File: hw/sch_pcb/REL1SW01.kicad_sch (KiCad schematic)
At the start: 22 parts, among them J1 HEADER_2x02_PARALLEL, J2 HEADER_2x02_PARALLEL, J3 HEADER_2x06_PARALLEL, J4 HEADER_2x06_PARALLEL, J5 HEADER_2x04_PARALLEL, M1 SROUB3M, M2 SROUB3M, M3 SROUB3M, M4 SROUB3M, T1 IRLML6244, T2 IRLML6244, X1 RELE

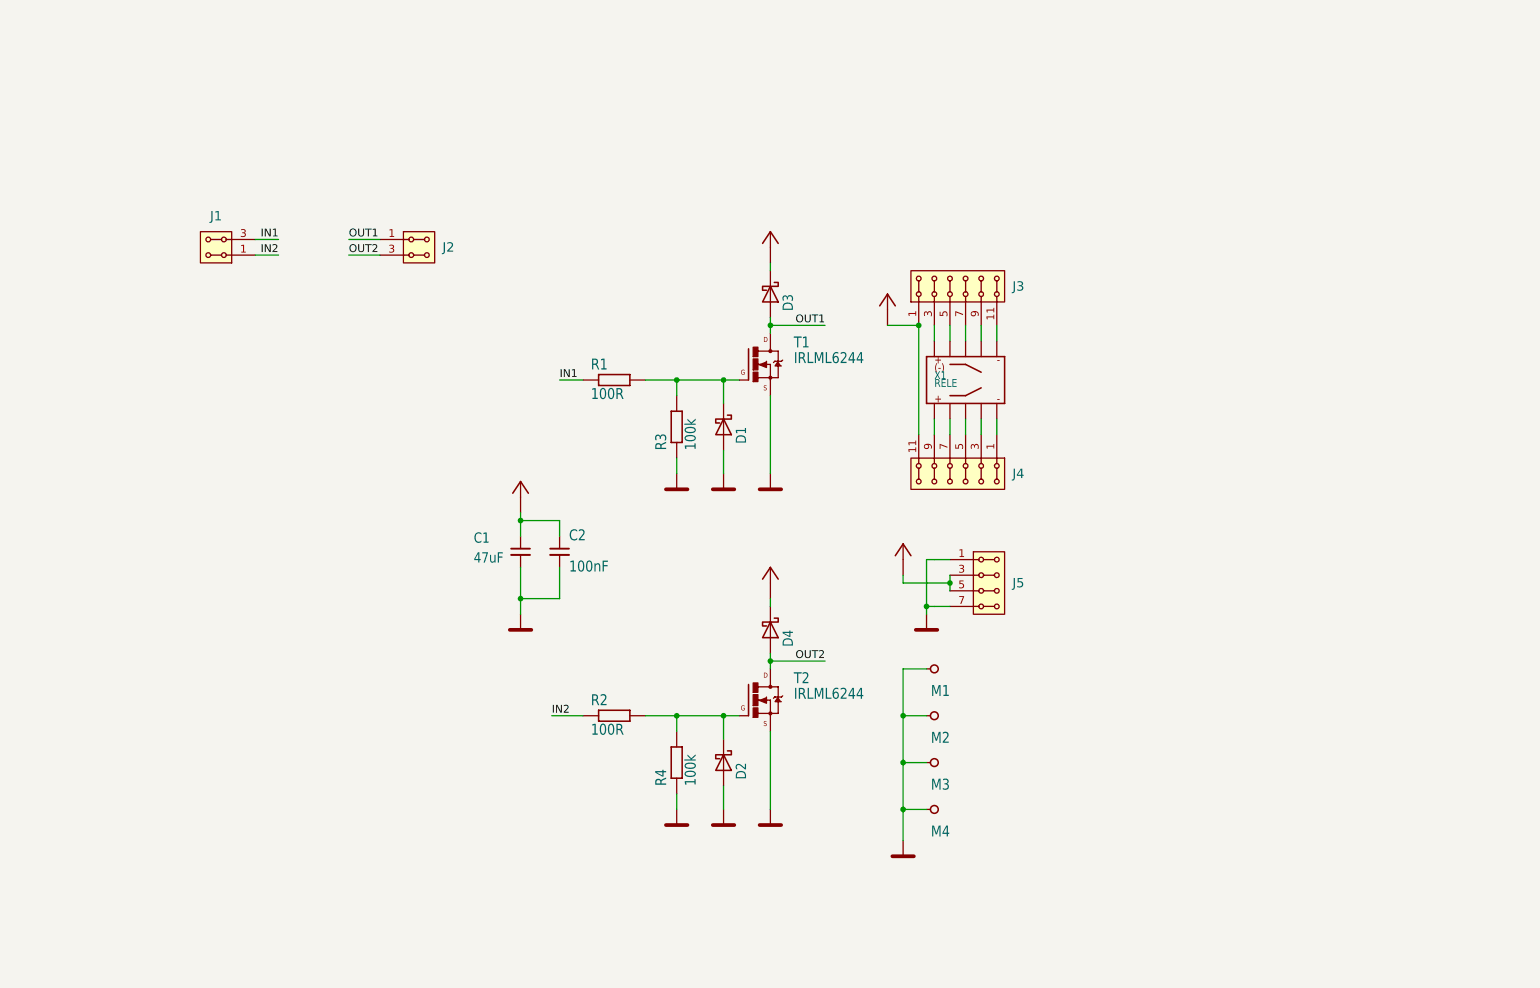
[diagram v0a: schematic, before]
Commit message: layout improvements
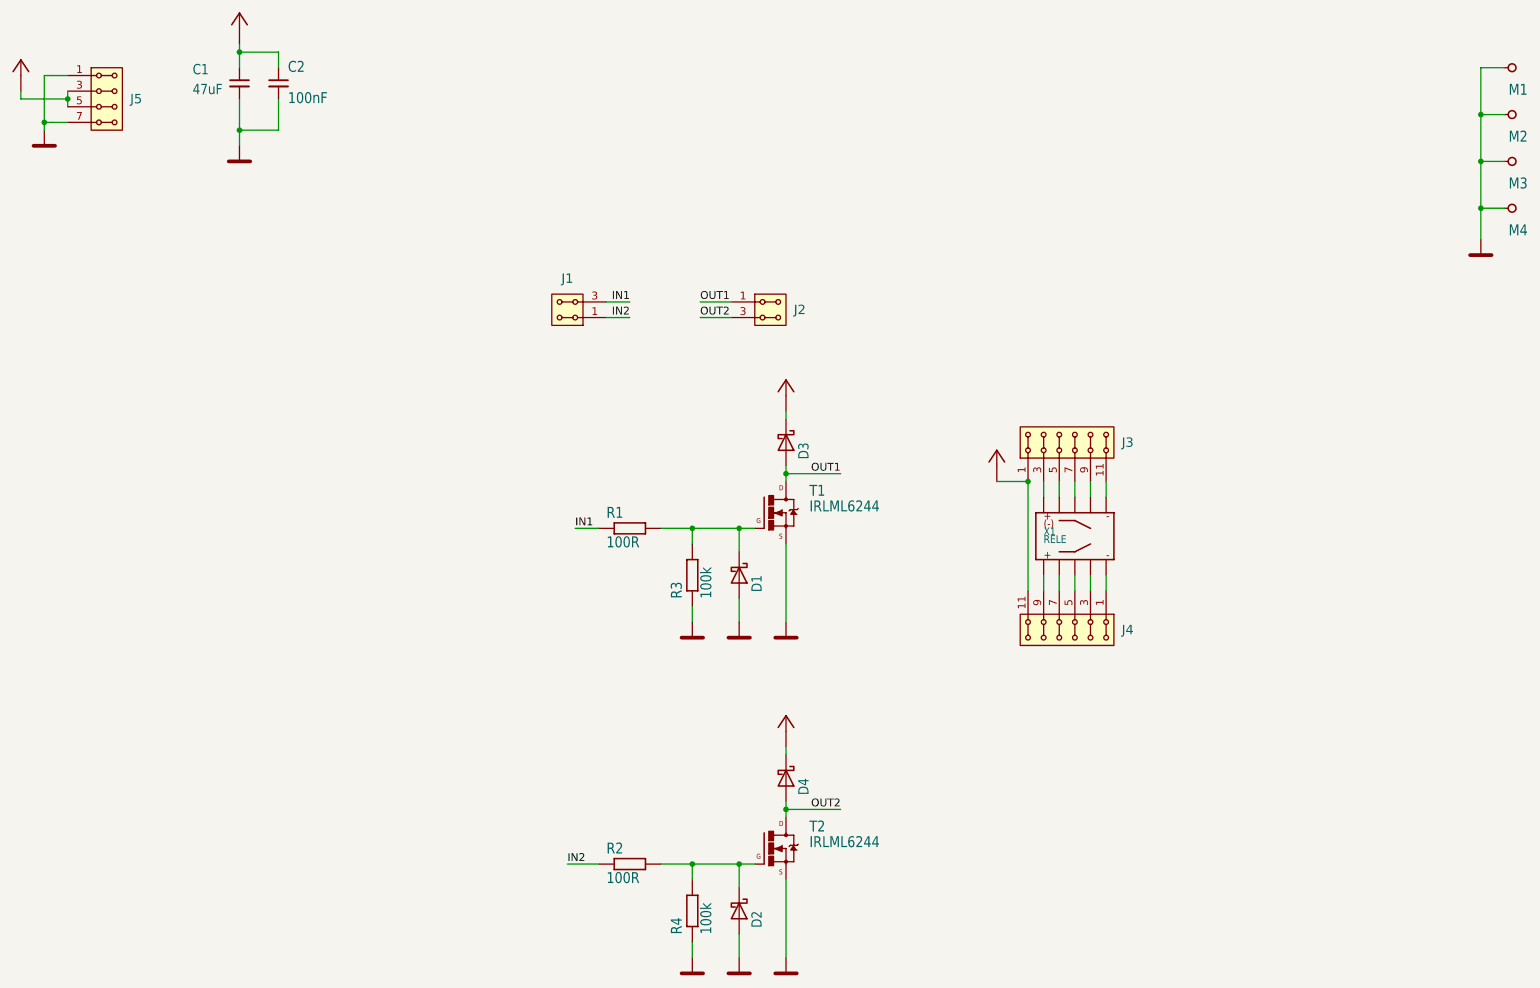
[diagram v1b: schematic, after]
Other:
- moved on the sheet: C1, C2, D1, D2, D3, D4, J1, J2, J3, J4, J5, M1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
